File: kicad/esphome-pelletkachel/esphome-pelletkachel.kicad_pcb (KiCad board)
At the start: 2 copper layers, 38.1 x 76.2 mm, 13 parts, among them J6 1-wire, U1 ESP32-DEVKITC-32U, U2 757

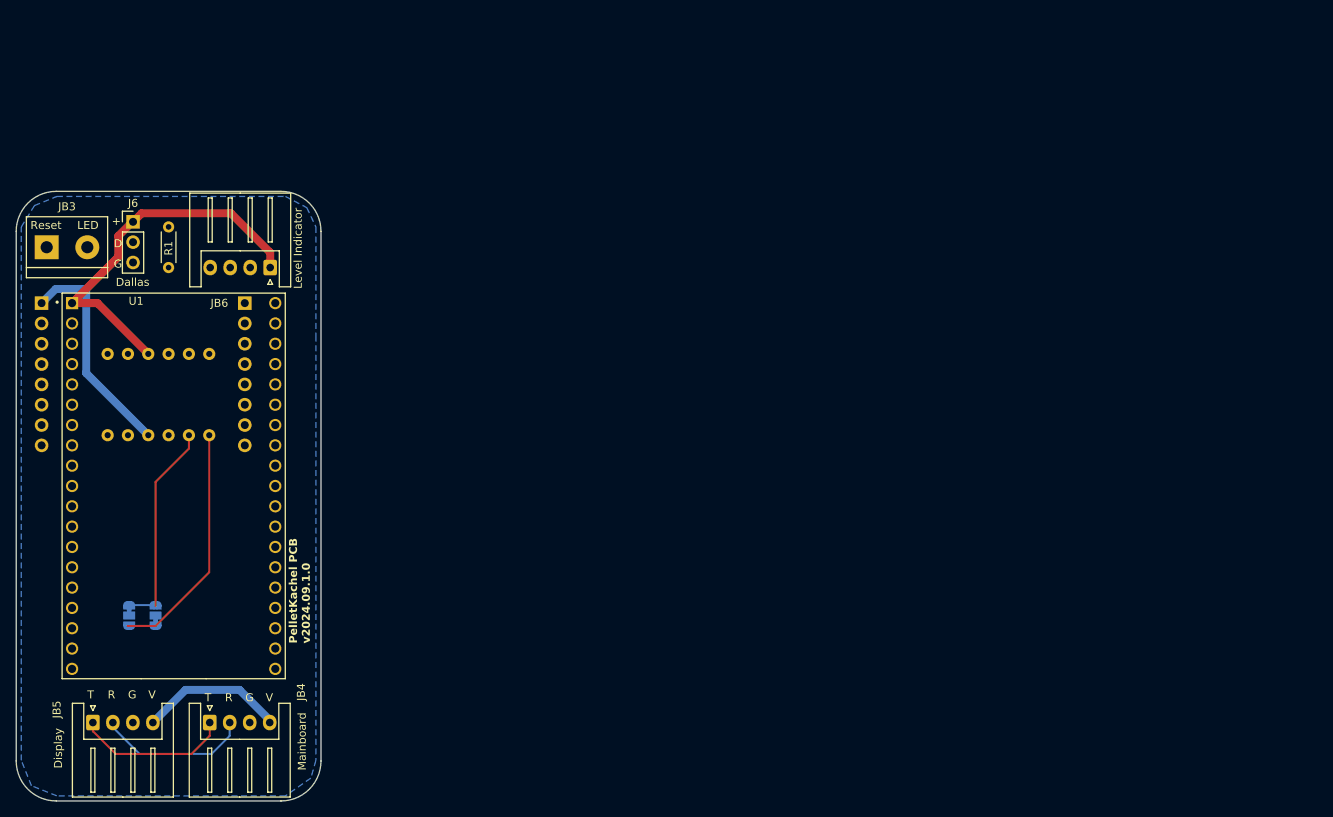
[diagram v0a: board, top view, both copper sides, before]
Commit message: gedoe
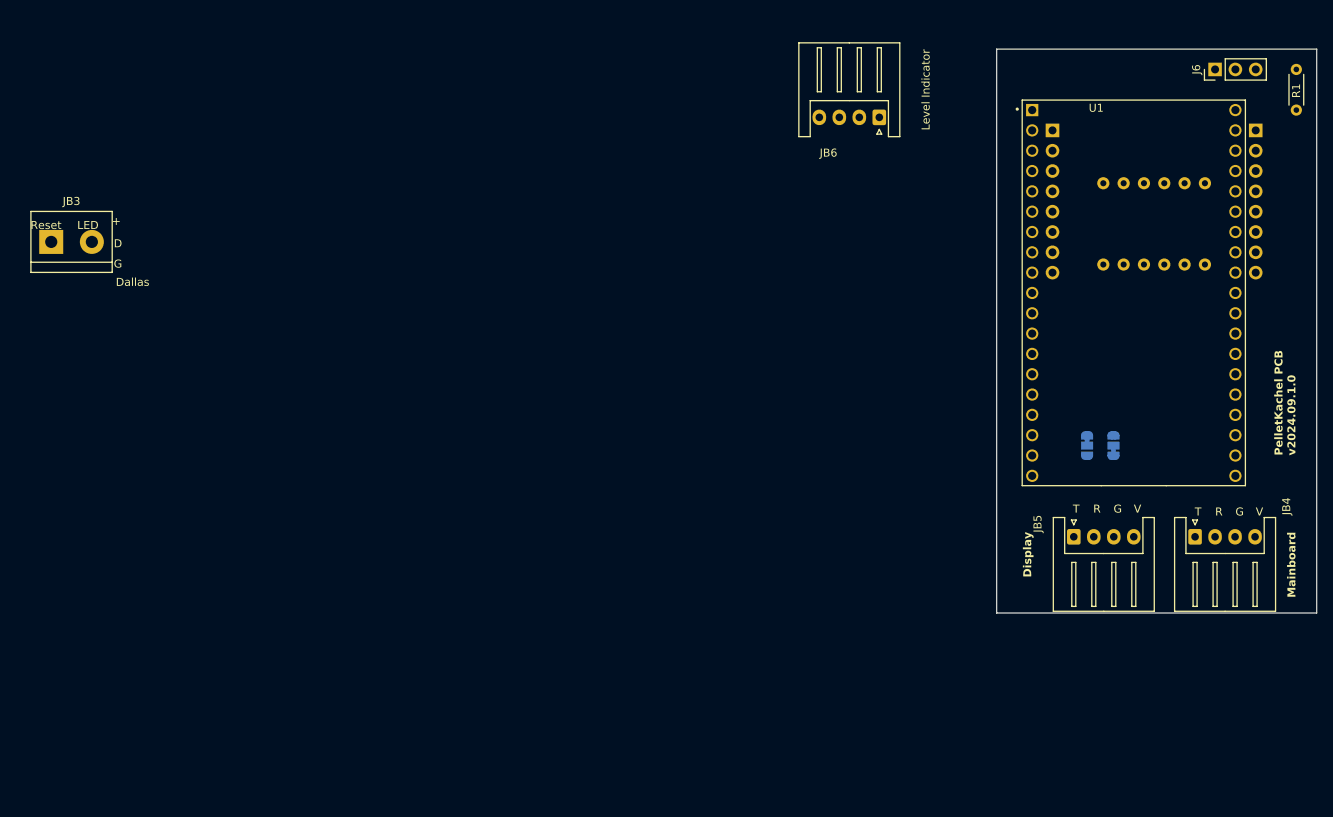
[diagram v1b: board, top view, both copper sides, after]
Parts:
- moved R1 142.3 mm to (228.6, 33.0)
- moved J6 136.6 mm to (218.4, 27.9), turned to 90 degrees
- moved JB1 128.2 mm to (198.1, 35.6)
- moved JB2 128.2 mm to (223.5, 35.6)
- moved U2 126.3 mm to (212.1, 59.9)
- moved JB4 125.3 mm to (215.9, 86.4)
- moved JB5 124.8 mm to (200.8, 86.4)
- moved U1 122.4 mm to (208.3, 55.9)
- moved G*** 122.2 mm to (213.4, 66.0)
- moved JP3 121.6 mm to (205.7, 75.0)
- moved JP2 121.6 mm to (202.4, 75.0)
- moved JB6 78.4 mm to (176.5, 33.9)
- moved JB3 0.88 mm to (73.0, 49.5)
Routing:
- net +3.3V: track 47.0 -> 0.00 mm
- net +5V: track 46.0 -> 0.00 mm
- net Net-(JP2-B): track 30.1 -> 0.00 mm
- net Net-(JP2-A): track 26.4 -> 0.00 mm
- net /MCUTX: track 19.5 -> 0.00 mm
- net /MCURX: track 19.2 -> 0.00 mm
- removed copper zone on B.Cu, net GND
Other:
- board size 38.1 x 76.2 mm -> 40 x 70.5 mm
